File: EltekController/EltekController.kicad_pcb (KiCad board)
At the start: 4 copper layers, 55 x 40 mm, 28 parts, among them J1 CANBUS, J2 Display, J3 USB_B_Micro, Q1 UMH3N, SW1 Reset, SW2 Boot, U1 ESP32-WROOM-32E, U2 CP2104-F03-GMR, U3 TJA1051T/3/1J, U4 XC6206P332MR

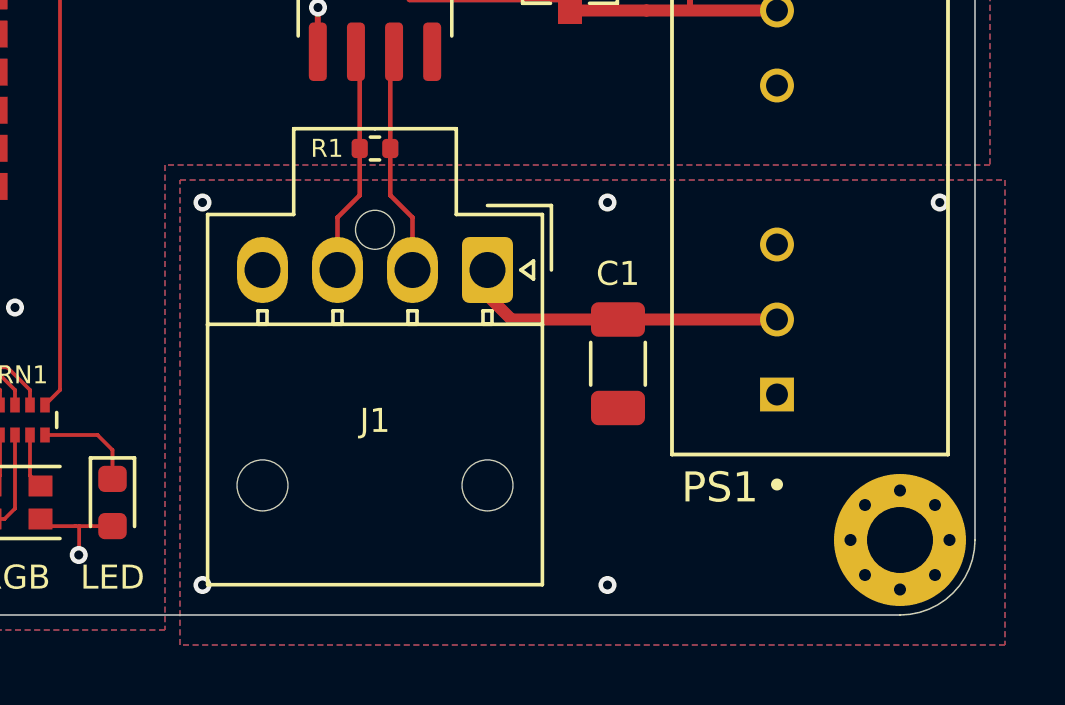
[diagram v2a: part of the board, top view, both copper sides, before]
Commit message: v0.1
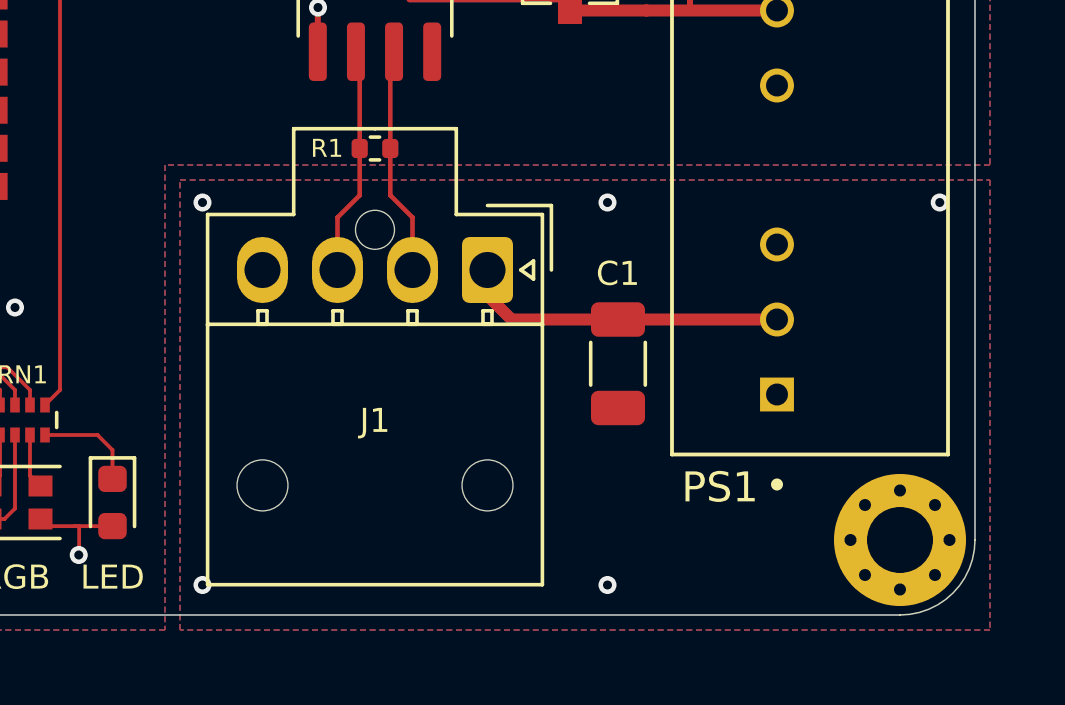
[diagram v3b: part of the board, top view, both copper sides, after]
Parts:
- renumbered JP2 to JP1

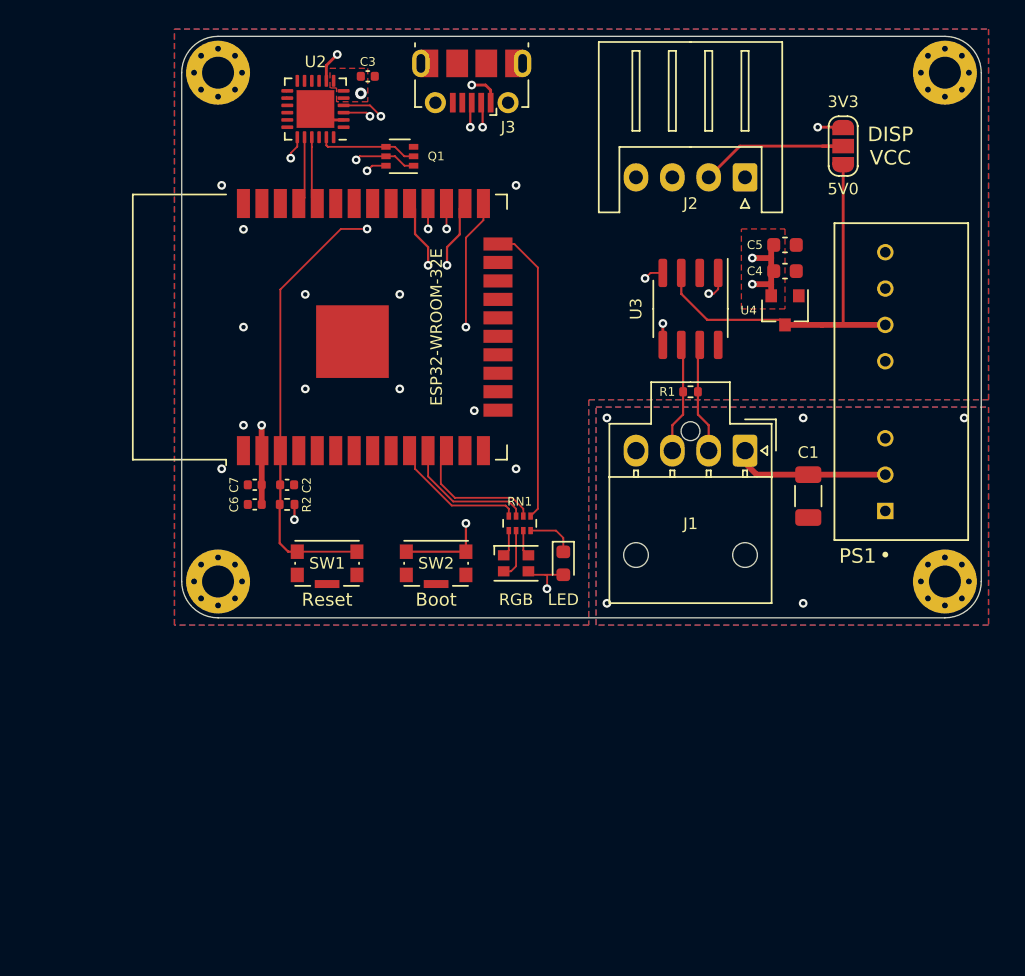
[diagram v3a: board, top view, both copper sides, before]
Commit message: Squashed commit of the following:
commit 90807526c89bbe23d0d14403179393f46968545b
Author: neg2led <4232981+neg2led@users.noreply.github.com>
Date:   Fri Feb 19 13:40:56 2021 +1100

    change vtabs

commit bdeb0cb4df280460f20d9cb7594185681e97bdea
Author: neg2led <4232981+neg2led@users.noreply.github.com>
Date:   Fri Feb 19 13:38:28 2021 +1100

    tiny tweak

commit 1e098ee4d97e67064c3c8c363f77a0e840b9e8c0
Author: neg2led <4232981+neg2led@users.noreply.github.com>
Date:   Fri Feb 19 13:37:41 2021 +1100

    almost...

commit b00c0a0b75bab0a44da9d349d5dc3fbb57f6d1e8
Author: neg2led <4232981+neg2led@users.noreply.github.com>
Date:   Fri Feb 19 01:39:59 2021 +1100

    and so it continues

reworked the whole dealio

almost...

tiny tweak

change vtabs
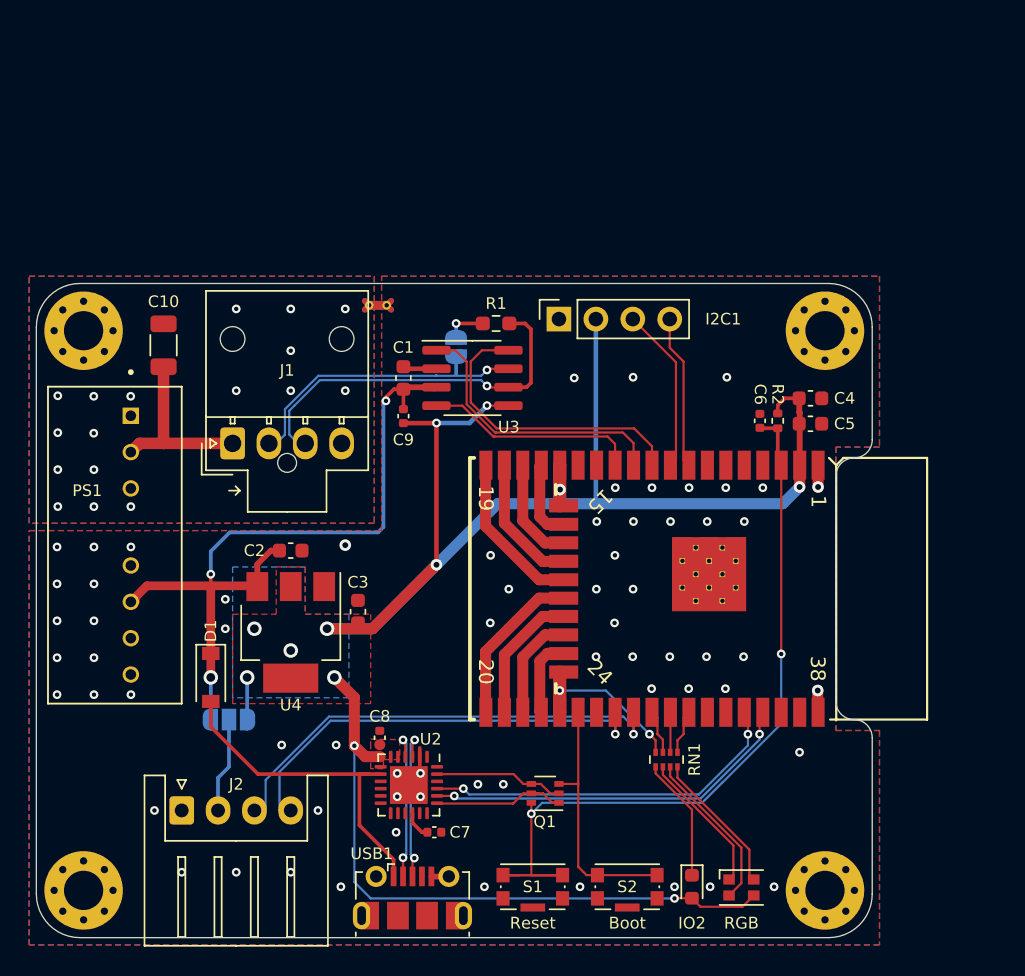
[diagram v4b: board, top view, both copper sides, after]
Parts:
- removed the C3 at (122.8, 62.8)
- removed J3: USB_B_Micro, Connector_USB:USB_Micro-B_Molex-105017-0001
- removed SW1: Reset, 1 My Footprints:SW_Push_1P1T-SH_NO_CK_KMR2xxG_3D
- removed SW2: Boot, 1 My Footprints:SW_Push_1P1T-SH_NO_CK_KMR2xxG_3D
- added C10: 1uF, Capacitor_SMD:C_1206_3216Metric, F.Cu at (108.8, 81.2)
- added C4: 22uF, Capacitor_SMD:C_0603_1608Metric, F.Cu at (153.2, 84.9)
- added C8: 10uF, Capacitor_SMD:C_0402_1005Metric, F.Cu at (123.6, 108.2)
- added C9: 100nF, Capacitor_SMD:C_0402_1005Metric, F.Cu at (125.2, 86.1)
- added D1: B5819W, Diode_SMD:D_SOD-123, F.Cu at (112.0, 104.1)
- added I2C1: OLED, Connector_PinSocket_2.54mm:PinSocket_1x04_P2.54mm_Vertical, F.Cu at (135.9, 79.5)
- added JP2: VJ2, Jumper:SolderJumper-3_P1.3mm_Open_RoundedPad1.0x1.5mm_NumberLabels, B.Cu at (113.2, 107.0)
- added LOGO1: Logo_Open_Hardware_Small, 1 My Footprints:neggle-logo-0.12, B.Cu at (145.0, 92.5)
- added NT1: GND_TIE, NetTie:NetTie-2_THT_Pad0.3mm, F.Cu at (124.1, 78.5)
- added S1: Reset, 1 My Footprints:SW_Push_1P1T-SH_NO_CK_KMR2xxG_3D, F.Cu at (134.2, 118.5)
- added S2: Boot, 1 My Footprints:SW_Push_1P1T-SH_NO_CK_KMR2xxG_3D, F.Cu at (140.7, 118.5)
- added USB1: USB-SER, Connector_USB:USB_Micro-B_Molex-105017-0001, F.Cu at (125.9, 119.2)
- C1: value 1uF -> 10uF; footprint Capacitor_SMD:C_1206_3216Metric -> Capacitor_SMD:C_0603_1608Metric
- C2: value 1uF -> 10uF; footprint Capacitor_SMD:C_0402_1005Metric -> Capacitor_SMD:C_0603_1608Metric
- C3: renamed from C4; value 10uF -> 22uF
- C5: value 1uF -> 100nF
- C6: value 10uF -> 1uF
- C7: value 1uF -> 4.7uF
- D3: renamed from D2; value LED -> IO2
- H1, H2, H3, H4: footprint MountingHole:MountingHole_2.2mm_M2_Pad_Via -> MountingHole:MountingHole_2.7mm_M2.5_Pad_Via
- JP1: value VDISP -> CAN_T; footprint Jumper:SolderJumper-3_P1.3mm_Open_RoundedPad1.0x1.5mm_NumberLabels -> Jumper:SolderJumper-2_P1.3mm_Open_RoundedPad1.0x1.5mm; moved to B.Cu
- R1: footprint Resistor_SMD:R_0402_1005Metric -> Resistor_SMD:R_0603_1608Metric_Pad0.98x0.95mm_HandSolder
- U1: footprint RF_Module:ESP32-WROOM-32 -> 1 My Footprints:ESP32-WROOM_WROVER_Dual_JLC_ManyVias
- U4: value XC6206P332MR -> AMS1117-3.3; footprint Package_TO_SOT_SMD:SOT-23 -> Package_TO_SOT_SMD:SOT-223-3_TabPin2
- moved J2 58.3 mm to (110.0, 113.2), turned to 0 degrees
- moved PS1 53.9 mm to (106.5, 93.8), turned to 270 degrees
- moved U2 46.9 mm to (125.6, 111.5), turned to 270 degrees
- moved Q1 45.0 mm to (135.0, 112.1)
- moved U4 40.6 mm to (117.5, 101.0)
- moved C3 37.6 mm to (122.1, 99.6), turned to 270 degrees
- moved J1 35.3 mm to (113.5, 88.0), turned to 90 degrees
- moved C6 35.2 mm to (149.8, 86.5), turned to 90 degrees
- moved R2 34.2 mm to (151.0, 86.5), turned to 90 degrees
- moved JP1 30.0 mm to (128.9, 81.4), turned to 270 degrees
- moved C1 29.0 mm to (125.2, 83.5)
- moved U1 28.8 mm to (145.0, 98.0), turned to 180 degrees
- moved D2 27.2 mm to (148.5, 118.5)
- moved C7 26.9 mm to (127.4, 114.8), turned to 180 degrees
- moved D3 23.9 mm to (145.1, 118.5)
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- renumbered D1 to D2
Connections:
- net /RXLED renamed Net-(U2-Pad13)
- net /TXLED renamed Net-(U2-Pad14)
- C1 pad 1: GNDPWR -> +5V
- C1 pad 2: +48V -> GND
- C2 pad 1: /~RST -> GND
- C2 pad 2: GND -> +5V
- C6 pad 1: GND -> /~RST
- C6 pad 2: +3V3 -> GND
- C7 pad 2: +3V3 -> Net-(C7-Pad2)
- D3 pad 1: Net-(D2-Pad1) -> Net-(D3-Pad1)
- H1 pad 1: GND -> GNDPWR
- H4 pad 1: GNDPWR -> GND
- JP1 pad 1: +5V -> Net-(JP1-Pad1)
- JP1 pad 2: Net-(J2-Pad2) -> /CAN+
- R1 pad 2: /CAN+ -> Net-(JP1-Pad1)
- RN1 pad 1: /R -> Net-(D3-Pad1)
- RN1 pad 2: /G -> /R
- RN1 pad 3: /B -> /G
- RN1 pad 4: Net-(D2-Pad1) -> /B
- RN1 pad 5: /LED_G2 -> /LED_B
- RN1 pad 6: /LED_B -> /LED_G
- RN1 pad 7: /LED_G -> /LED_R
- RN1 pad 8: /LED_R -> /GPIO2_LED
- U1 pad 10: /LED_R -> /CAN_S
- U1 pad 11: /LED_G -> /CAN_TX
- U1 pad 12: /LED_B -> /CAN_RX
- U1 pad 24: /LED_G2 -> /GPIO2_LED
- U1 pad 26: /CAN_RX -> Net-(U1-Pad26)
- U1 pad 29: /CAN_TX -> /LED_R
- U1 pad 30: Net-(U1-Pad30) -> /LED_G
- U1 pad 31: Net-(U1-Pad31) -> /LED_B
- U1 pad 8: Net-(U1-Pad8) -> /OLED_SDA
- U1 pad 9: Net-(U1-Pad9) -> /OLED_SCL
- U2 pad 16: Net-(U2-Pad16) -> Net-(C7-Pad2)
- U3 pad 8: Net-(U3-Pad8) -> /CAN_S
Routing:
- net +3V3: track 19.1 -> 132.1 mm, vias 8 -> 11
- net +5V: track 27.4 -> 51.6 mm, vias 0 -> 3
- net /~RST: track 36.2 -> 58.0 mm
- net /UART_TX: track 4.73 -> 25.9 mm, vias 0 -> 2
- net /CAN_S: track 0.00 -> 20.7 mm
- net /LED_G2: track 20.7 -> 0.00 mm
- net /UART_RX: track 4.72 -> 25.3 mm, vias 0 -> 2
- net /CAN-: track 7.63 -> 26.8 mm, vias 0 -> 1
- net /D_RXSDA: track 16.2 -> 30.2 mm
- net /CAN+: track 7.63 -> 21.5 mm, vias 0 -> 1
- net /D_TXSCL: track 20.6 -> 32.3 mm
- net /GPIO2_LED: track 0.00 -> 11.6 mm, vias 0 -> 2
- net /OLED_SCL: track 0.00 -> 11.4 mm
- net Net-(U1-Pad20): track 0.00 -> 11.1 mm
- net Net-(U1-Pad19): track 0.00 -> 11.1 mm
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- added copper zone on B.Cu, net +3V3
- removed copper zone on In2.Cu, net +3V3
- removed copper zone on In1.Cu, net GND
- removed copper zone on In1.Cu, net GNDPWR
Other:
- board size 55 x 40 mm -> 57.5 x 45 mm
- copper layers 4 -> 2
- net class USB_D added: clearance 0.1524, trace_width 0.1524, via_dia 0.6, via_drill 0.3
- net class VIN: clearance 0.4 -> 0.254
- board text added: "Origin X=100mm, Y=77mm"
- board text removed: "DISP VCC"
